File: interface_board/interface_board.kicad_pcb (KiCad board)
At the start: 2 copper layers, 41.9 x 111.5 mm, 38 parts, among them J1 FPGA_devboard, J2 5V_PWR, J3 Serial IEEE-488 Bus, J4 IBM PC floppy disk drive conn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, Q1 BC337, U1 74LS06, U2 74LVC14, U3 74LS06, U4 74LVC14

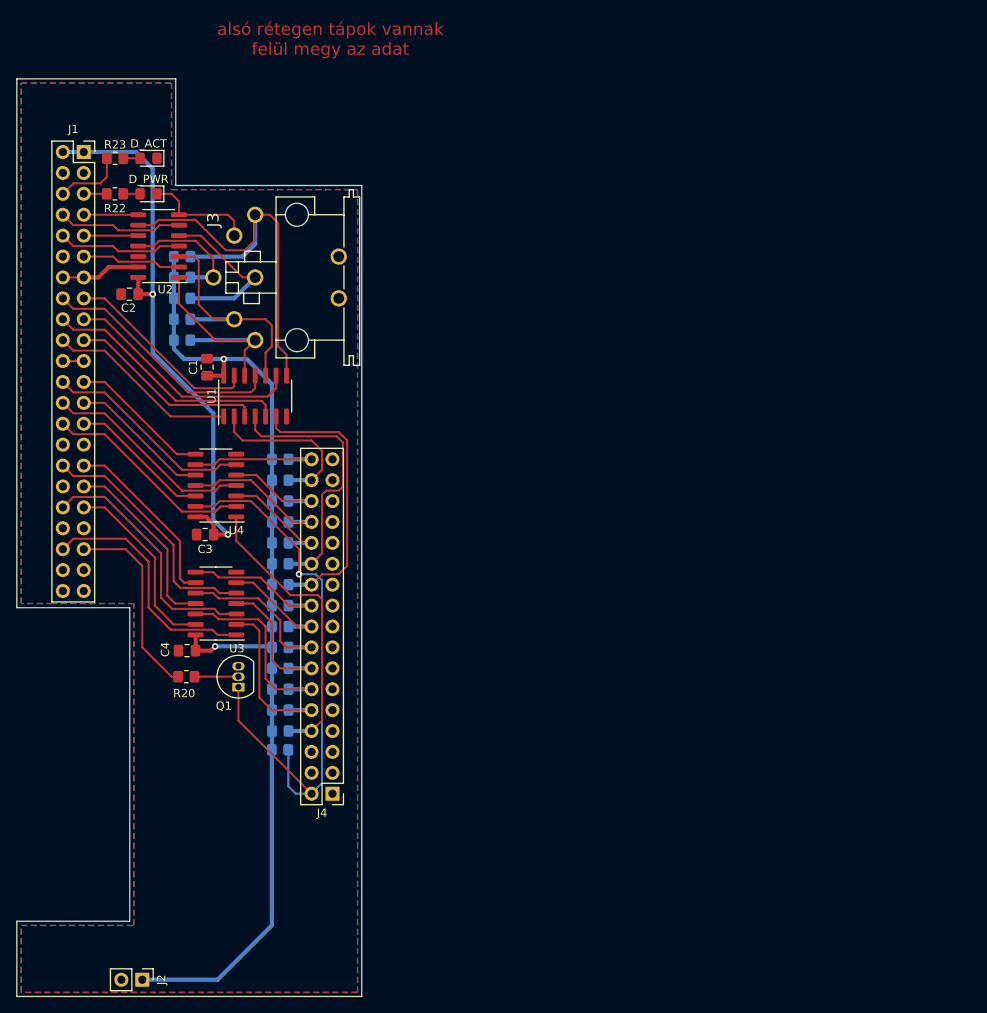
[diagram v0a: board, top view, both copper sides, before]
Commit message: Finish interface board PCB
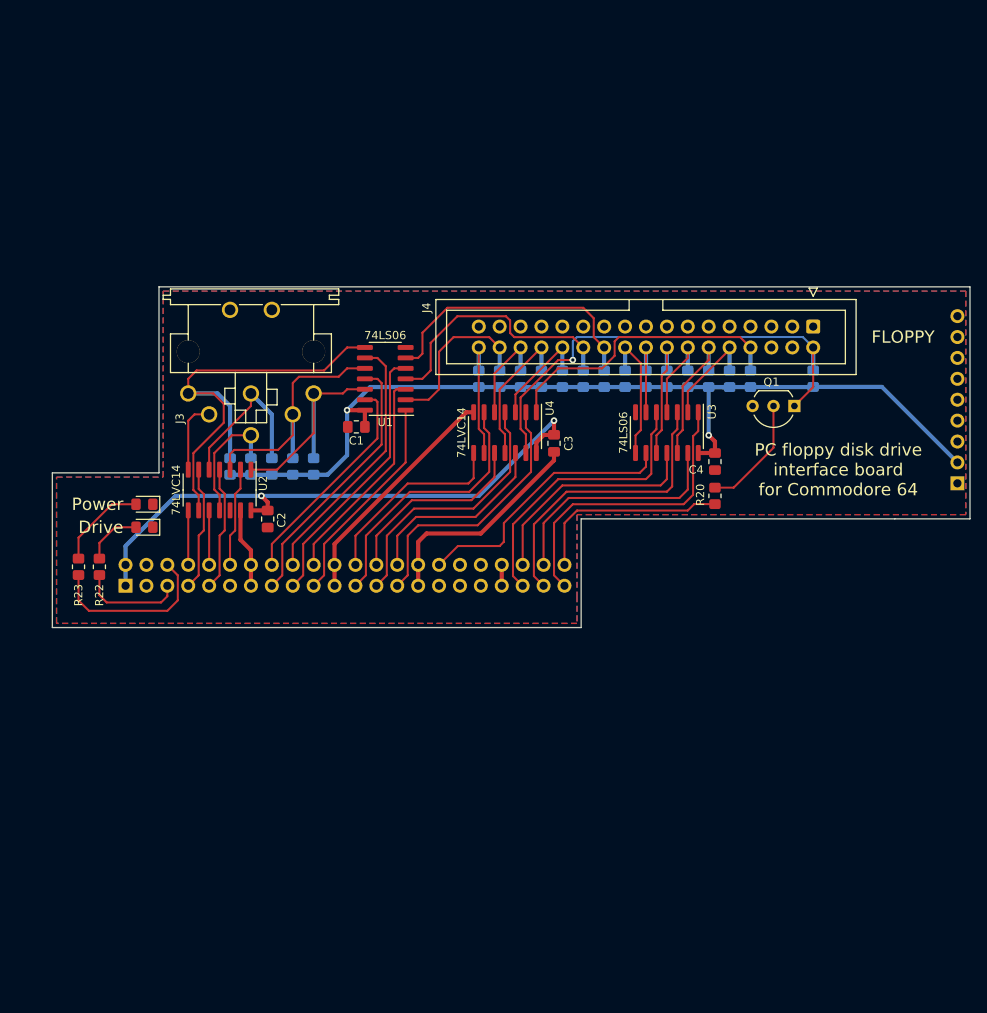
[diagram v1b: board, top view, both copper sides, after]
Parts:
- removed D_ACT: GREEN, LED_SMD:LED_0805_2012Metric_Pad1.15x1.40mm_HandSolder
- removed D_PWR: RED, LED_SMD:LED_0805_2012Metric_Pad1.15x1.40mm_HandSolder
- added D_ACT1: GREEN, LED_SMD:LED_0805_2012Metric_Pad1.15x1.40mm_HandSolder, F.Cu at (104.4, 104.0)
- added D_PWR1: RED, LED_SMD:LED_0805_2012Metric_Pad1.15x1.40mm_HandSolder, F.Cu at (104.4, 101.2)
- J1: moved to B.Cu
- J2: footprint Connector_PinHeader_2.54mm:PinHeader_1x02_P2.54mm_Vertical -> Connector_PinHeader_2.54mm:PinHeader_1x09_P2.54mm_Vertical; moved to B.Cu
- J4: footprint Connector_PinHeader_2.54mm:PinHeader_2x17_P2.54mm_Vertical -> Connector_IDC:IDC-Header_2x17_P2.54mm_Vertical
- Q1: footprint Package_TO_SOT_THT:TO-92_Inline -> Package_TO_SOT_THT:TO-92_Inline_Wide
- moved J2 116.0 mm to (203.2, 98.7), turned to 0 degrees
- moved J4 81.5 mm to (185.7, 79.6), turned to -90 degrees
- moved R21 78.9 mm to (185.7, 86.0), turned to 90 degrees
- moved Q1 75.7 mm to (183.4, 89.3), turned to 180 degrees
- moved R13 71.4 mm to (178.1, 86.0), turned to 90 degrees
- moved C4 68.1 mm to (173.7, 96.0), turned to -90 degrees
- moved R20 67.9 mm to (173.7, 100.2), turned to 90 degrees
- moved R6 67.8 mm to (175.5, 86.0), turned to 90 degrees
- moved R7 64.3 mm to (173.0, 86.0), turned to 90 degrees
- moved R8 60.7 mm to (170.4, 86.0), turned to 90 degrees
- moved U3 58.6 mm to (167.9, 92.5), turned to -90 degrees
- moved R9 57.2 mm to (167.9, 86.0), turned to 90 degrees
- moved R10 53.7 mm to (165.4, 86.0), turned to 90 degrees
- moved J1 52.9 mm to (102.1, 111.1), turned to -90 degrees
- moved R11 50.2 mm to (162.8, 86.0), turned to 90 degrees
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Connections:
- J1 pad 10: /CLK_IN -> /RESET_IN
- J1 pad 11: /DATA_IN -> unconnected-(J1-Pad11)
- J1 pad 12: unconnected-(J1-Pad12) -> /DATA_IN
- J1 pad 15: /DATA_OUT -> /CLK_OUT
- J1 pad 16: /CLK_OUT -> /DATA_OUT
- J1 pad 17: /SRQ_OUT -> /WDATE
- J1 pad 18: /WDATE -> /SRQ_OUT
- J1 pad 19: /WGATE -> /SIDE1
- J1 pad 20: /SIDE1 -> /WGATE
- J1 pad 23: /DSKCHG -> /RDATA
- J1 pad 24: /RDATA -> /DSKCHG
- J1 pad 25: /WPT -> /TRK00
- J1 pad 26: /TRK00 -> /WPT
- J1 pad 27: /REDWC_IN -> /INDEX
- J1 pad 28: /INDEX -> /REDWC_IN
- J1 pad 31: /STEP -> unconnected-(J1-Pad31)
- J1 pad 32: /DIR -> /STEP
- J1 pad 33: /MOTEB -> unconnected-(J1-Pad33)
- J1 pad 35: /DRVSB -> unconnected-(J1-Pad35)
- J1 pad 36: /DRVSA -> unconnected-(J1-Pad36)
- J1 pad 39: /REDWC_OUT -> /DIR
- J1 pad 40: /MOTEA -> /MOTEB
- J1 pad 41: unconnected-(J1-Pad41) -> /DRVSA
- J1 pad 42: unconnected-(J1-Pad42) -> /DRVSB
- J1 pad 43: unconnected-(J1-Pad43) -> /MOTEA
- J1 pad 44: unconnected-(J1-Pad44) -> /REDWC_OUT
- J1 pad 5: /PWR -> /ACTION
- J1 pad 6: /ACTION -> /PWR
- J1 pad 7: /SQR_IN -> /ATN_IN
- J1 pad 8: /ATN_IN -> /SQR_IN
- J1 pad 9: /RESET_IN -> /CLK_IN
- J2 pad 1: +5V -> GND
- J2 pad 2: GND -> +5V
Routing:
- net GND: track 25.7 -> 76.6 mm
- net /PWR: track 2.79 -> 21.0 mm
- net /IBM PC floppy interface/~{REDWC}: track 72.1 -> 58.3 mm
- net /STEP: track 22.2 -> 33.1 mm
- net Net-(D_PWR1-Pad2): track 2.06 -> 11.2 mm
- net Net-(Q1-Pad2): track 5.33 -> 14.2 mm
- net /IBM PC floppy interface/~{MOTEA}: track 21.0 -> 12.8 mm
- net +5V: track 124.7 -> 116.7 mm
- net /IBM PC floppy interface/~{DRVSB}: track 24.4 -> 17.2 mm
- net /MOTEA: track 29.7 -> 36.8 mm
- net /DSKCHG: track 17.2 -> 23.9 mm
- net /WPT: track 17.2 -> 23.8 mm
- net /TRK00: track 25.7 -> 32.3 mm
- net /REDWC_IN: track 17.2 -> 23.8 mm
- net /INDEX: track 25.7 -> 32.3 mm
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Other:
- board size 41.9 x 111.5 mm -> 111.5 x 41.4 mm
- board text added: "Drive"
- board text added: "FLOPPY"
- board text added: "JLCJLCJLCJLC"
- board text added: "PC floppy disk drive interface board for Commodore 64"
- board text added: "Power"
- board text added: "SERIAL"
- board text added: "Weisz Pál 2022"
- board text removed: "JTAG"
- board text removed: "alsó rétegen tápok vannak felül megy az adat"
